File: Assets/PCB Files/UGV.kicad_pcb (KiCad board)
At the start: 2 copper layers, 200.1 x 192.5 mm, 74 parts, among them J1 B2B-XH-A, J10 B2B-XH-A, J11 B2B-XH-A, J12 B2B-XH-A, J13 USB3_A, J14 B2B-XH-A, J15 Screw_Terminal_01x12, J16 Screw_Terminal_01x12, J17 Screw_Terminal_01x12, J18 Screw_Terminal_01x12, J19 XT90PW-M, J20 XT30PW-M, J21 XT30PW-M, J23 B2B-XH-A, J24 XT30PW-M, J25 XT30PW-M, J26 XT30PW-M, J30 B2B-XH-A, J32 B2B-XH-A, J33 B2B-XH-A, J34 XT30PW-M, J35 XT30PW-M, J36 B2B-XH-A, J37 XT30PW-M, J39 XT30PW-M, J4 B4B-XH-A_LF__SN_, J40 B2B-XH-A, J41 B2B-XH-A, J42 B2B-XH-A, J43 B2B-XH-A, J44 B4B-XH-A_LF__SN_, J45 B4B-XH-A_LF__SN_, J46 B4B-XH-A_LF__SN_, J47 B4B-XH-A_LF__SN_, J5 B2B-XH-A, J6 B2B-XH-A, J7 B2B-XH-A, J8 B2B-XH-A, J9 B2B-XH-A, U1 INA219AxDCN, U2 LMR33630ADDA, U3 SN74LVC8T245, U4 Teensy4.1, U5 SN74LVC8T245

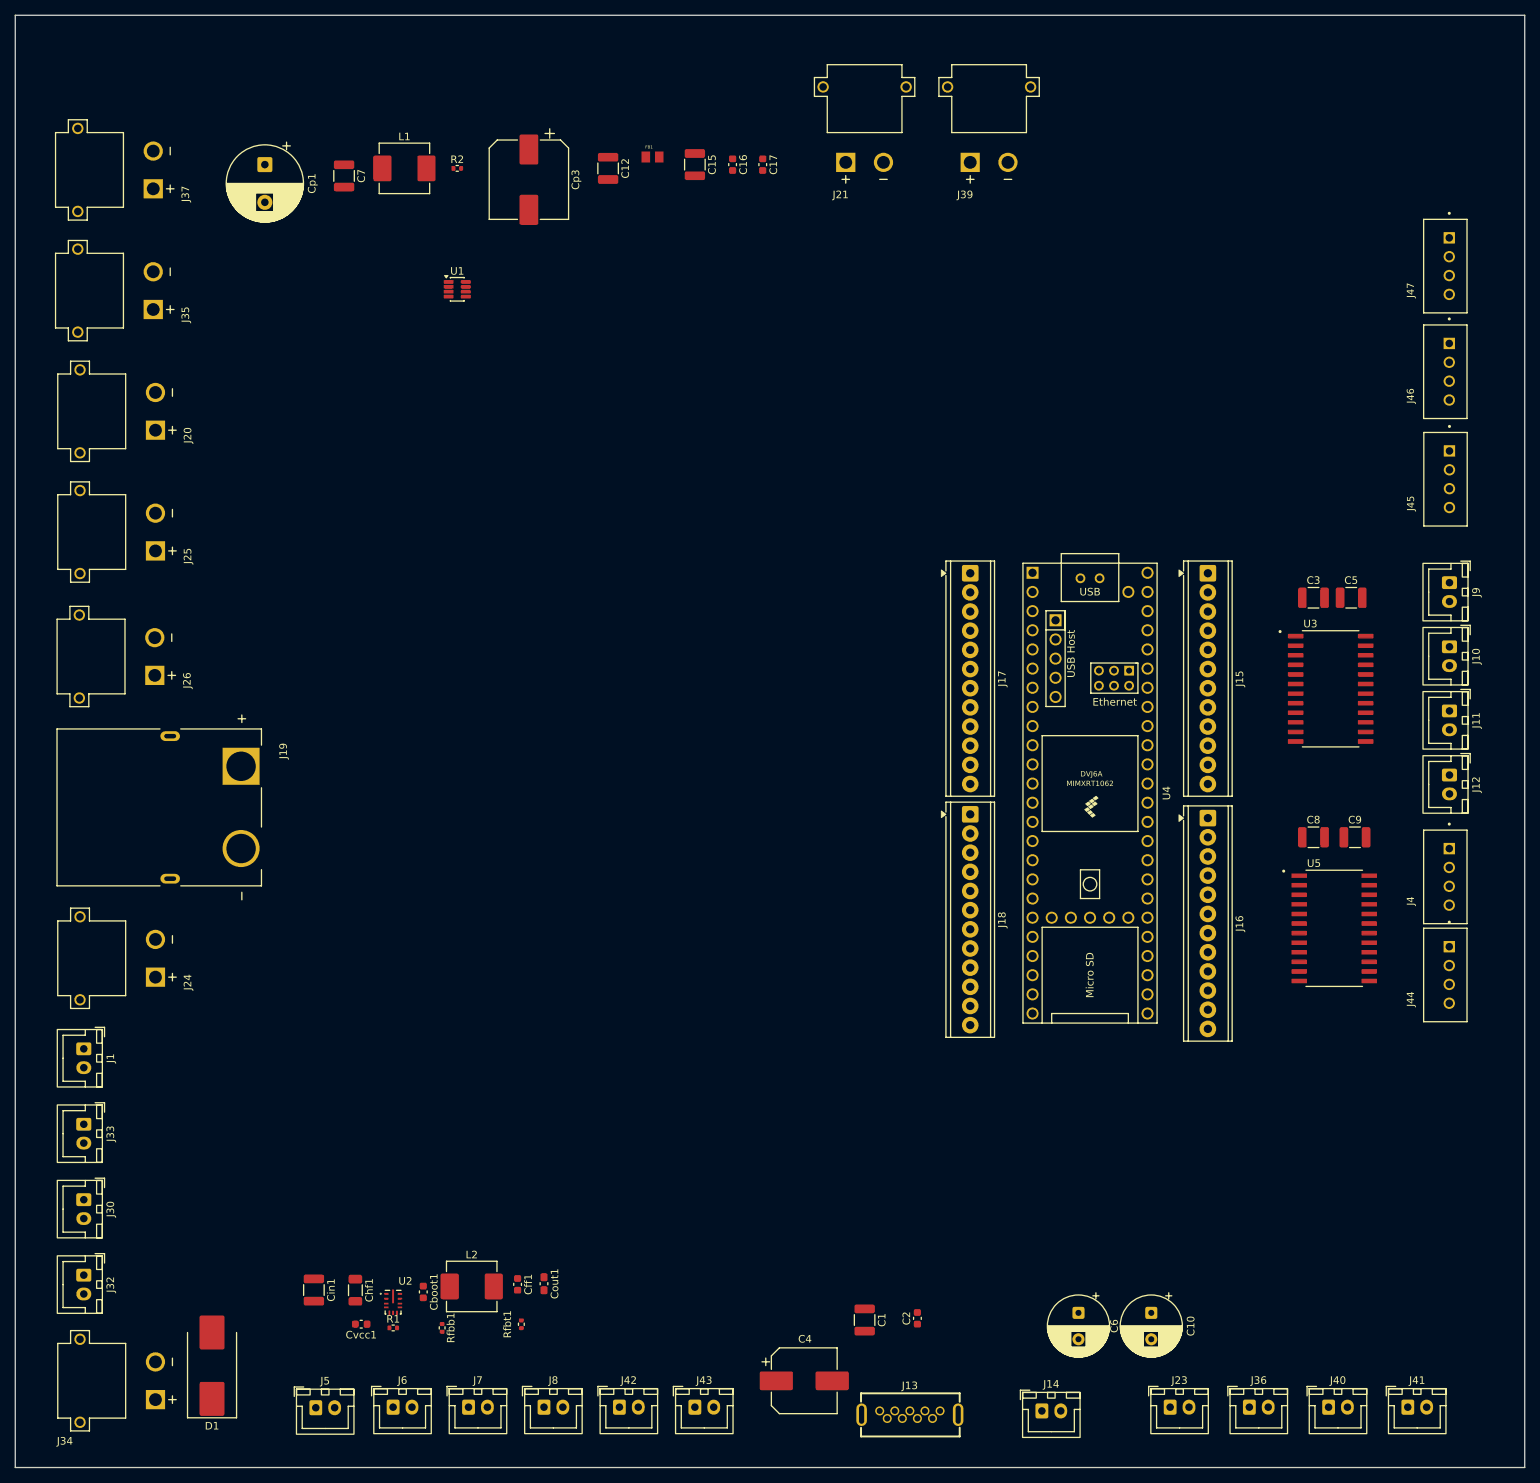
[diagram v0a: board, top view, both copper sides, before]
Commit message: PCB updated
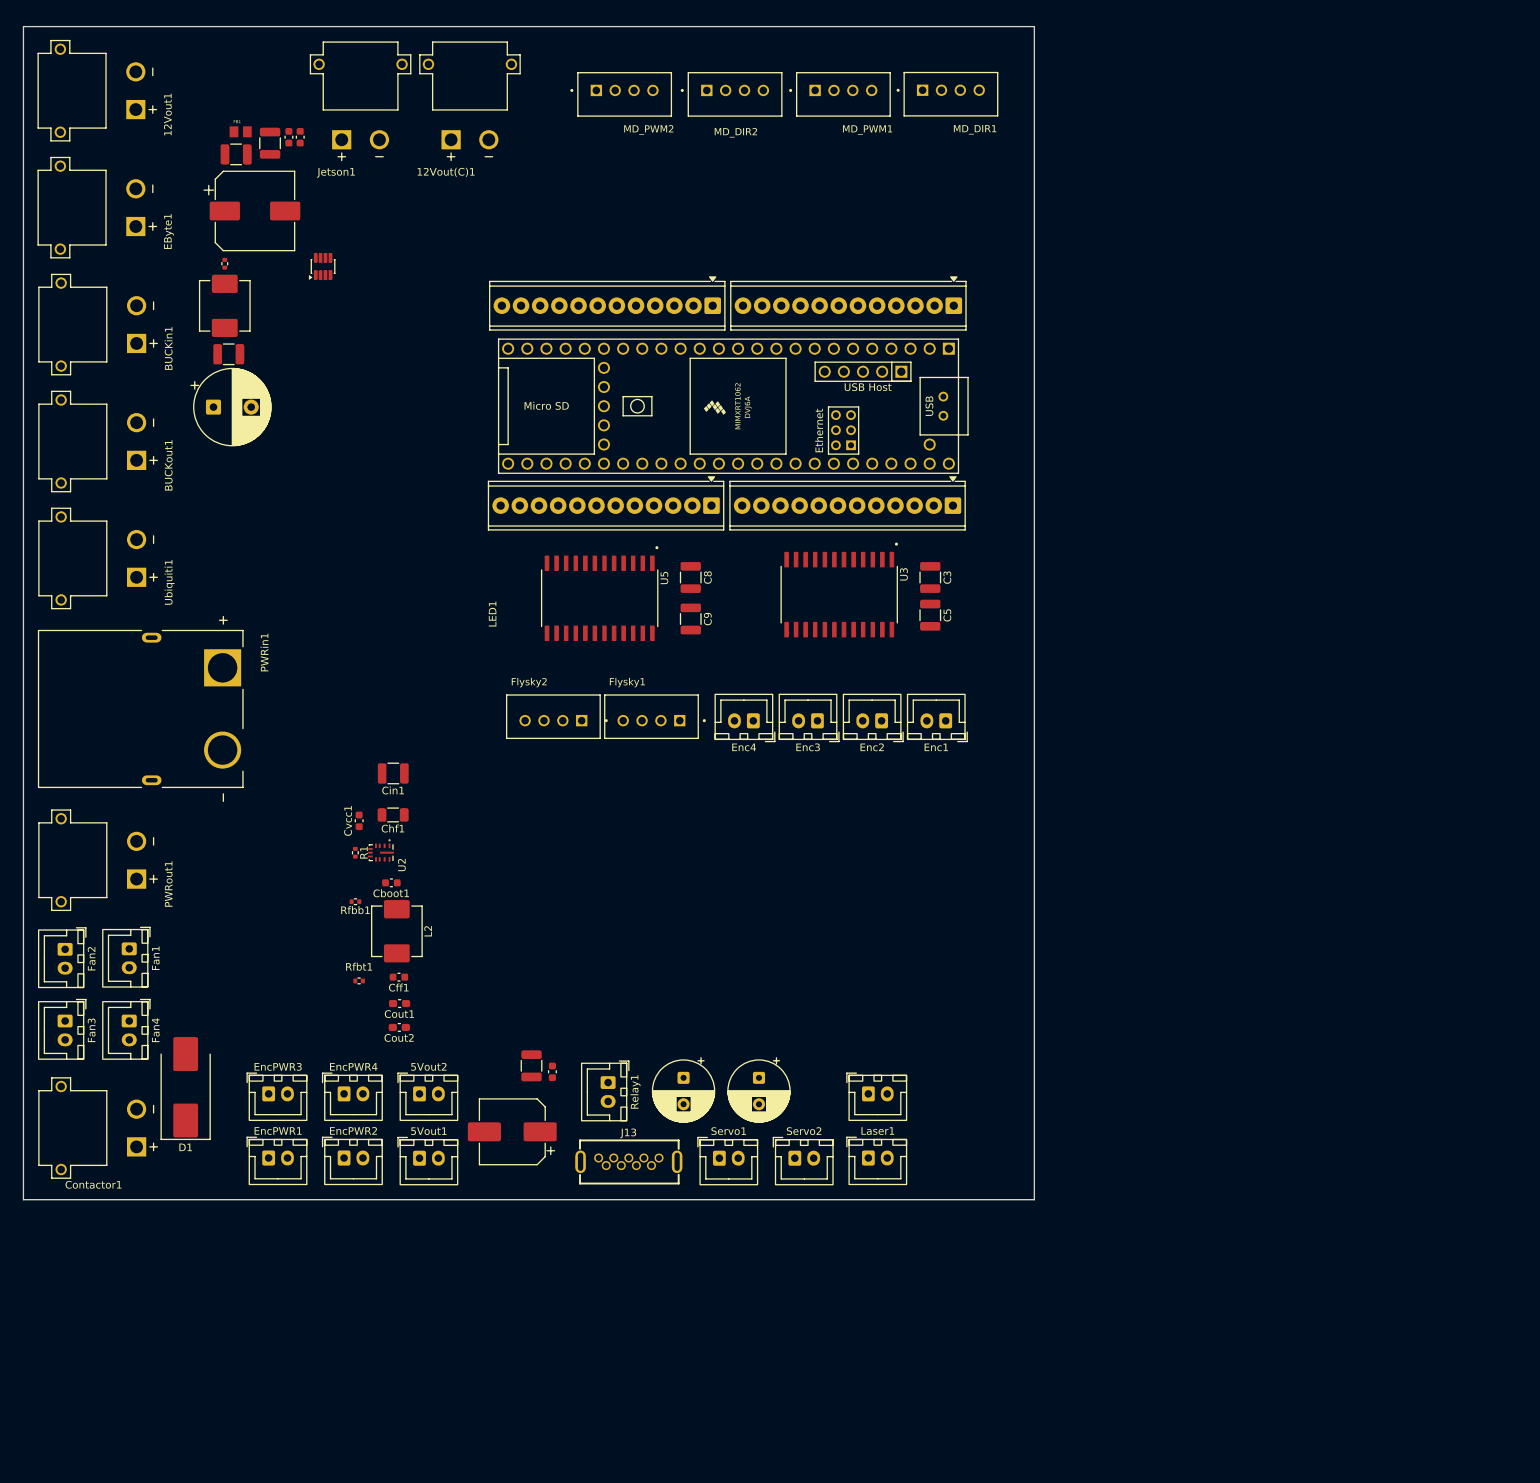
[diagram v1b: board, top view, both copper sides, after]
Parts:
- added Cout2: 22uF, Capacitor_SMD:C_0603_1608Metric_Pad1.08x0.95mm_HandSolder, F.Cu at (50.8, 134.2)
- added MD_PWM2: B4B-XH-A_LF__SN_, B4B-XH-A_LF__SN_:JST_B4B-XH-A_LF__SN_, F.Cu at (80.7, 10.5)
- Cout1: value 2 x 22uF -> 22uF
- R2: value 0.001 -> 0.01
- moved Flysky2 123.1 mm to (71.2, 93.0), turned to 0 degrees
- moved Flysky1 107.3 mm to (84.2, 93.0), turned to 0 degrees
- moved U5 106.7 mm to (77.4, 77.3), turned to -90 degrees
- moved MD_DIR2 96.9 mm to (95.3, 10.5), turned to 180 degrees
- moved C9 92.7 mm to (89.5, 80.0), turned to -90 degrees
- moved Enc4 92.6 mm to (97.8, 93.5), turned to 180 degrees
- moved C8 89.4 mm to (89.5, 74.5), turned to -90 degrees
- moved MD_PWM1 87.8 mm to (109.7, 10.5), turned to 180 degrees
- moved Enc3 83.8 mm to (106.2, 93.5), turned to 180 degrees
- moved MD_DIR1 83.1 mm to (123.9, 10.5), turned to 180 degrees
- moved Laser1 78.8 mm to (113.0, 151.5)
- moved J16 77.8 mm to (92.2, 65.0), turned to 180 degrees
- moved Enc2 75.9 mm to (114.8, 93.5), turned to 180 degrees
- moved J18 75.6 mm to (92.4, 38.5), turned to 180 degrees
- moved LED1 73.8 mm to (113.0, 143.0)
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- renumbered J39 to 12Vout(C)1, J37 to 12Vout1, J42 to 5Vout1, J43 to 5Vout2, J20 to BUCKin1, J25 to BUCKout1, J34 to Contactor1, J35 to EByte1, J9 to Enc1, J10 to Enc2, J11 to Enc3, J12 to Enc4, J8 to EncPWR1, J6 to EncPWR2, J5 to EncPWR3, J7 to EncPWR4, J1 to Fan1, J33 to Fan2, J30 to Fan3, J32 to Fan4, J4 to Flysky1, J44 to Flysky2, J21 to Jetson1, J40 to LED1, J41 to Laser1, J45 to MD_DIR1, J47 to MD_DIR2, J46 to MD_PWM1, J19 to PWRin1, J24 to PWRout1, J14 to Relay1, J23 to Servo1, J36 to Servo2, J26 to Ubiquiti1
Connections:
- C4 pad 1: GND -> /Vout
- C4 pad 2: /Vout -> GND
- R2 pad 1: Net-(U1-IN-) -> Net-(U1-IN+)
- R2 pad 2: Net-(U1-IN+) -> Net-(U1-IN-)
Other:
- board size 200.1 x 192.5 mm -> 134 x 155.5 mm
